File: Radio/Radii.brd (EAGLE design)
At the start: 42.6 x 44.3 mm, 55 parts, among them J1 10118193-0001LF, J2 BUTTON, J3 BUTTON, J4 BUTTON, J5 BUTTON, J6 BUTTON, U2 ATMEGA32U4-AU, U3 AP63203WU-7, U4 IND_1255AY-3R9N=P3, Y1 ECS-80-20-5PX-TR

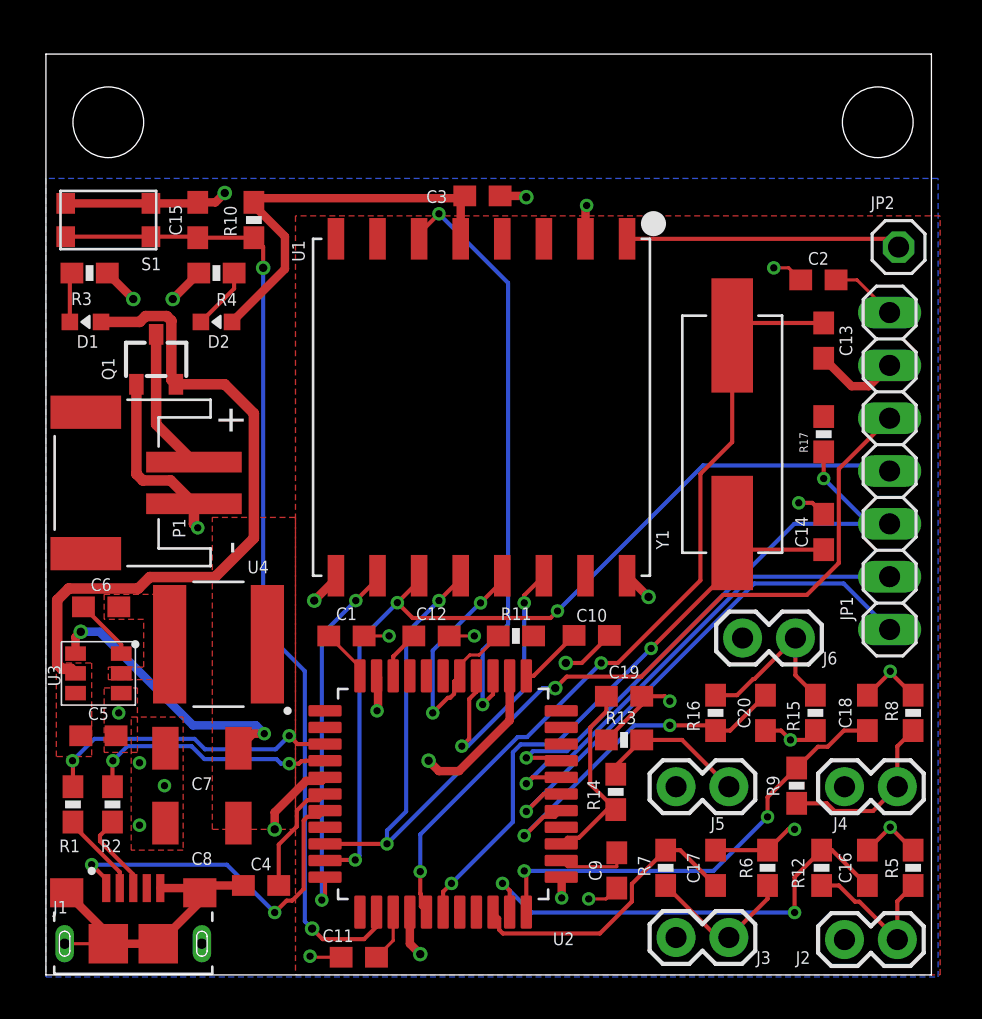
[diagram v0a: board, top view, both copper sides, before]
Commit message: Updated drill holes
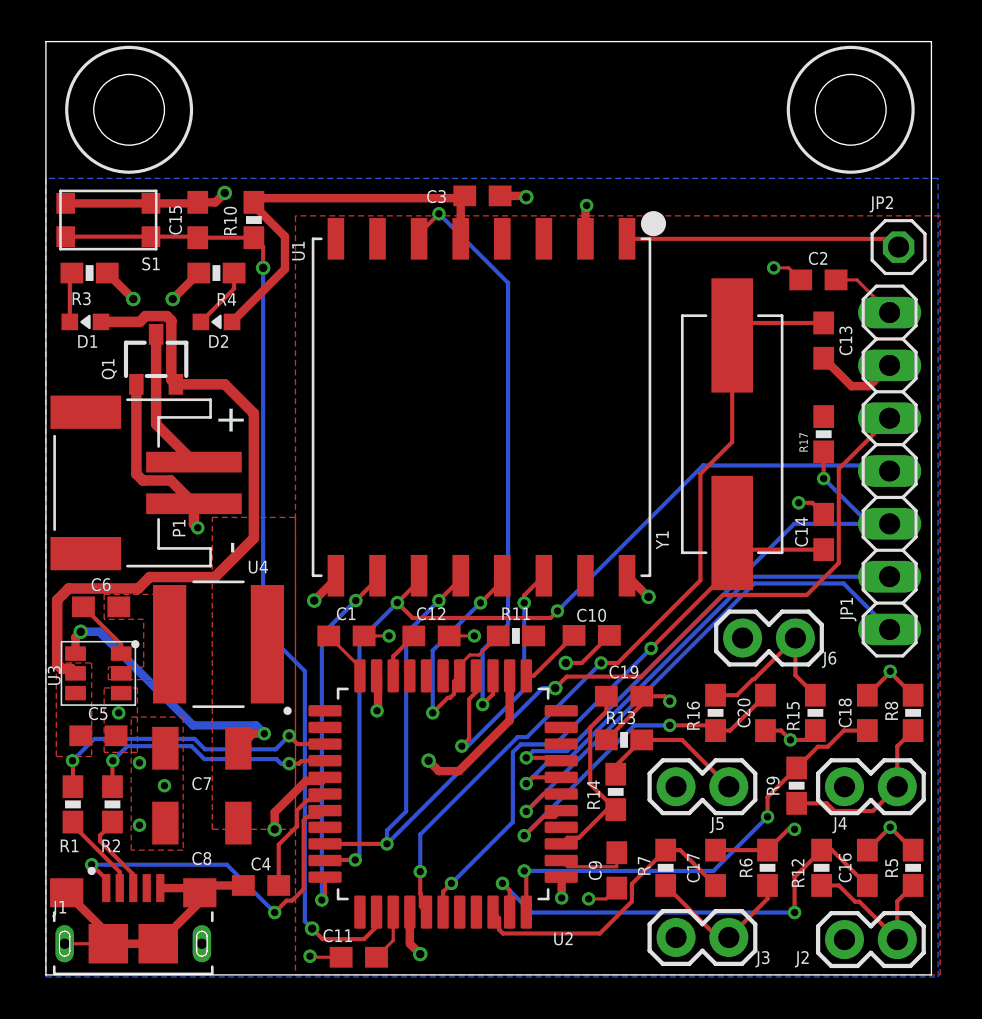
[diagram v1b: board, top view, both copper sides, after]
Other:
- board size 42.6 x 44.3 mm -> 42.6 x 44.9 mm
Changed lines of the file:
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@@
 <plain>
 <wire x1="0" y1="0" x2="42.58" y2="0" width="0" layer="20"/>
-<wire x1="42.58" y1="0" x2="42.58" y2="44.28" width="0" layer="20"/>
-<wire x1="42.58" y1="44.28" x2="0" y2="44.28" width="0" layer="20"/>
-<wire x1="0" y1="44.28" x2="0" y2="0" width="0" layer="20"/>
-<hole x="3" y="41" drill="3.4"/>
-<hole x="40" y="41" drill="3.4"/>
+<wire x1="42.58" y1="0" x2="42.58" y2="44.88" width="0" layer="20"/>
+<wire x1="42.58" y1="44.88" x2="0" y2="44.88" width="0" layer="20"/>
+<wire x1="0" y1="44.88" x2="0" y2="0" width="0" layer="20"/>
+<hole x="4" y="41.6" drill="3.4"/>
+<hole x="38.7" y="41.6" drill="3.4"/>
+<circle x="4" y="41.6" radius="3" width="0.1524" layer="21"/>
+<circle x="38.7" y="41.6" radius="3" width="0.1524" layer="21"/>
 </plain>
 <attributes>
